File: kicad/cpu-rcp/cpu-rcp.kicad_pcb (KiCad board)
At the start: 4 copper layers, 90.2 x 57.1 mm, 79 parts, among them P1 RDRAM-EDGE, P5 502790-5091, SW1 Reset, U10 CPU-NUS, U3 U3, U6 PIF-NUS, U7 MX8330, U8 LC125, U9 RCP-NUS, X1 14.318MHz

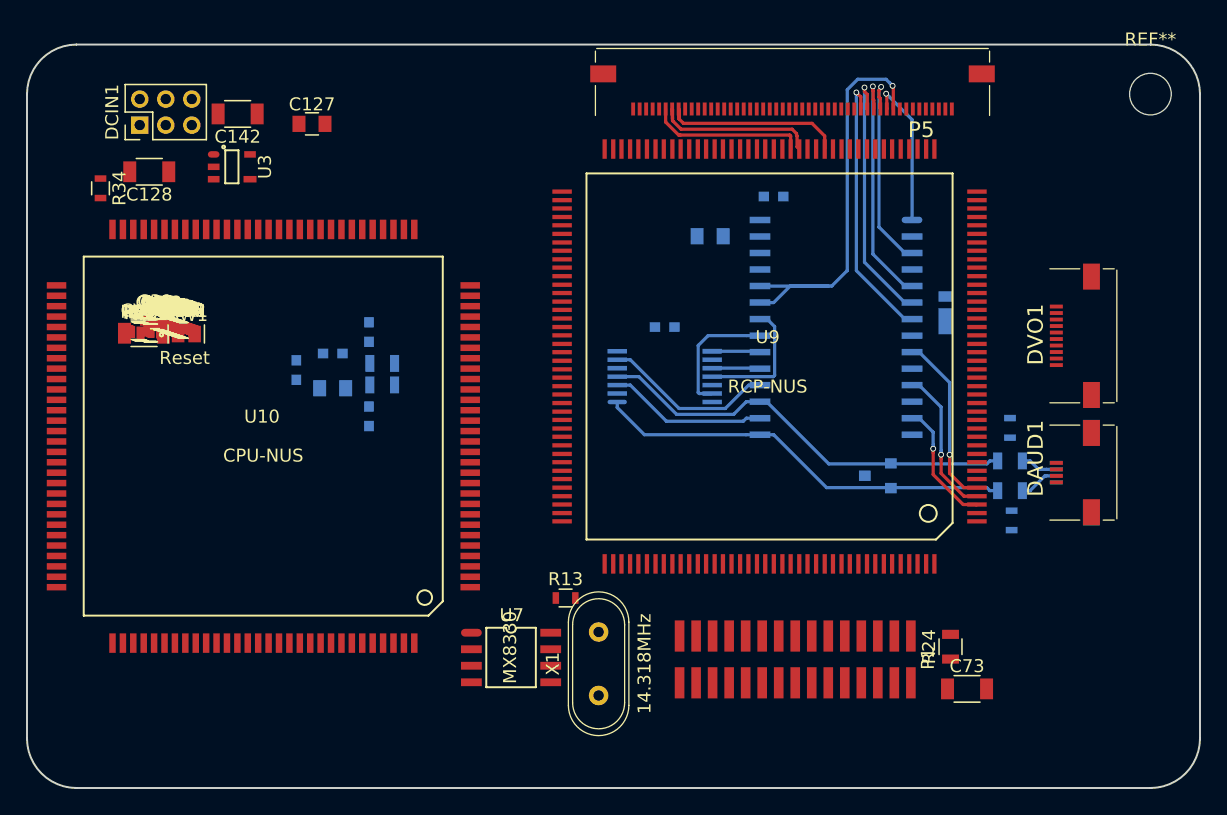
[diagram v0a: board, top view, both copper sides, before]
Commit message: WIP
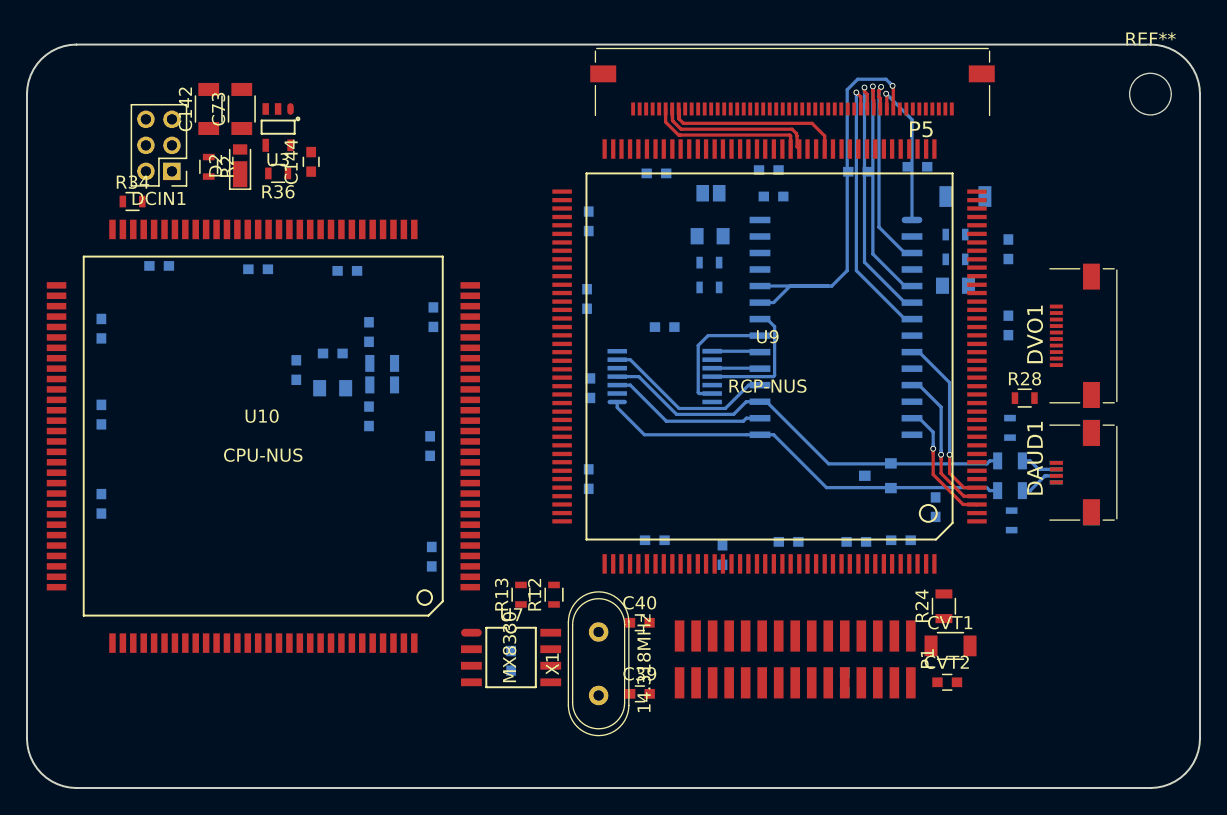
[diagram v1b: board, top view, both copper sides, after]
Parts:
- removed CU1: .1uF, n64:C_0603
- C127, C128, CC1, CC2, CC3, CC4, CC5, CC6, CC7, CC8, CC9, CR1, CR10, CR11, CR12, CR13, CR14, CR15, CR2, CR3, CR4, CR5, CR6, CR7, CR8, CR9, CU7, CVR1, CVR2, R22, R23, R3, R4, SW1: moved to B.Cu
- D2: moved to F.Cu
- moved C73 71.4 mm to (41.9, 30.4), turned to 90 degrees
- moved R28 68.2 mm to (102.1, 52.6)
- moved CVT2 66.6 mm to (96.1, 74.4)
- moved CVT1 66.5 mm to (96.4, 71.6)
- moved CR2 65.4 mm to (100.8, 47.0), turned to 270 degrees
- moved CR3 64.4 mm to (100.8, 41.1), turned to 270 degrees
- moved R3 63.2 mm to (96.8, 40.0)
- moved R4 62.9 mm to (96.8, 41.9)
- moved C128 62.8 mm to (97.5, 37.1), turned to 0 degrees
- moved CR1 59.9 mm to (95.2, 61.0), turned to 90 degrees
- moved CR15 57.9 mm to (92.6, 63.5)
- moved CR4 57.8 mm to (93.9, 34.8)
- moved CVR1 57.6 mm to (88.3, 74.4), turned to 270 degrees
- moved D2 55.4 mm to (41.8, 34.4)
- moved CR14 54.4 mm to (89.2, 63.6)
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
